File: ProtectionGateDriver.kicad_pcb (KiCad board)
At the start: 2 copper layers, 46.2 x 33.3 mm, 19 parts, among them J1 48V_INPUT_XT_MALE, J2 WHEEL_OUTPUT_XT_FEMALE, J3 12V_GATE_SUPPLY, J4 STM_CONTROL, Q1 MCTL1D0N08Y, U1 1EDN7550B

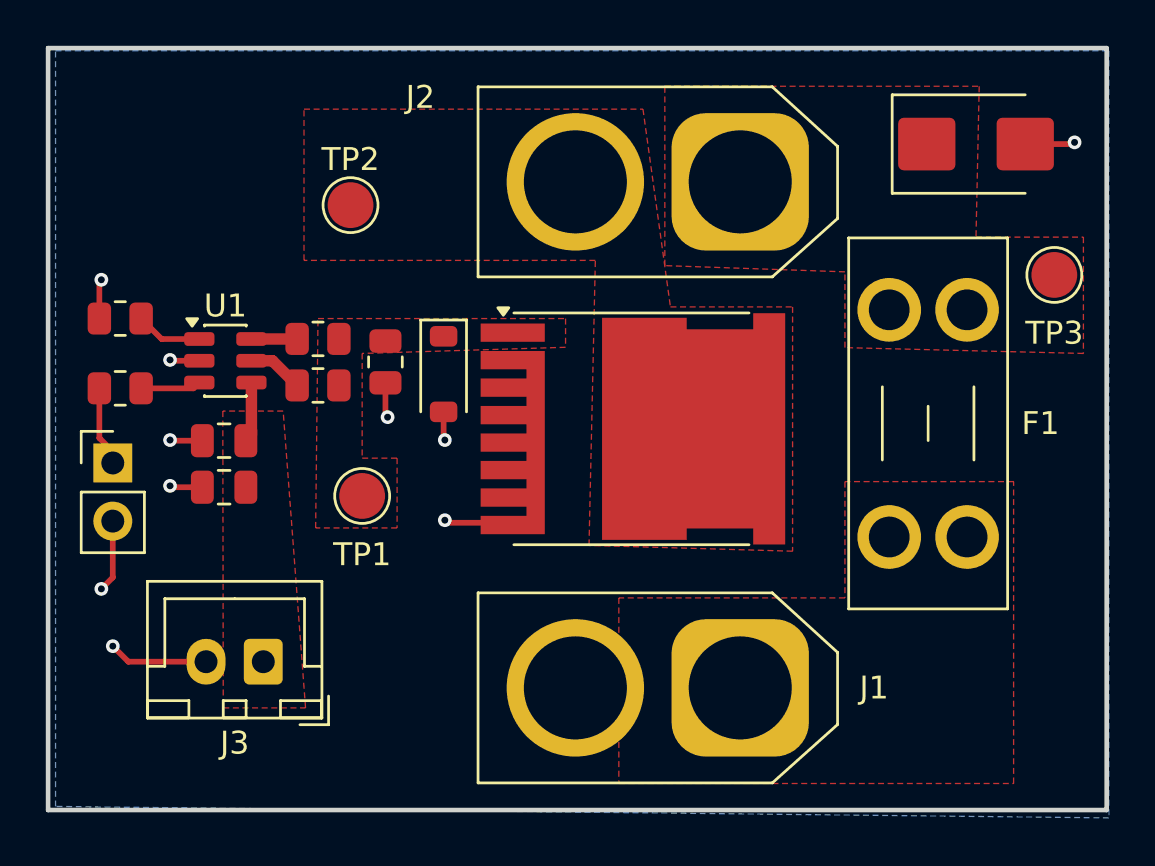
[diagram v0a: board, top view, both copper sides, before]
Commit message: Correct iteration 2 native KiCad files from uploaded project
Replace stale PCB, project and schematic with the supplied iteration 2 files. Four-layer layout is a review checkpoint, not for fabrication.
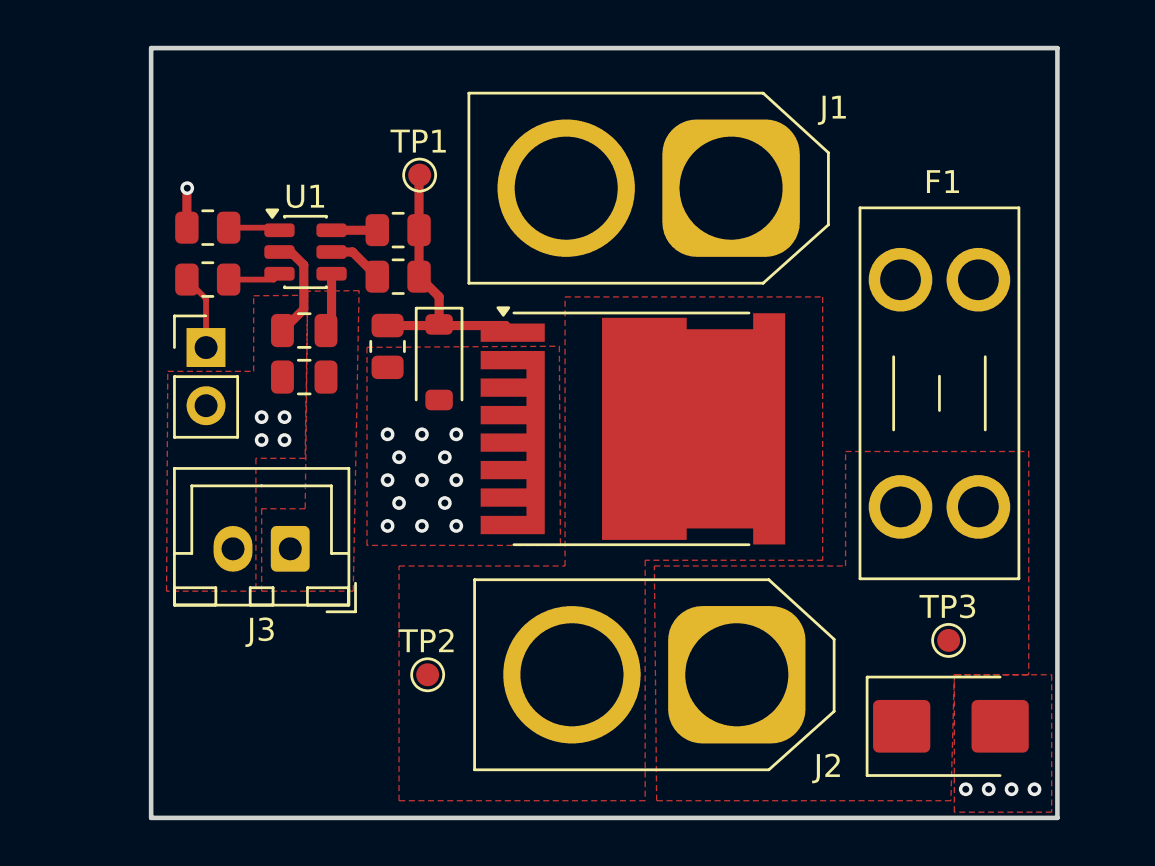
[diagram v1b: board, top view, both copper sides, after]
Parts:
- TP1, TP2, TP3: footprint TestPoint:TestPoint_Pad_D2.0mm -> TestPoint:TestPoint_Pad_D1.0mm
- moved D2 25.4 mm to (161.6, 109.5)
- moved J1 21.8 mm to (152.0, 86.0)
- moved J2 21.5 mm to (152.2, 107.2)
- moved TP2 20.8 mm to (138.8, 107.2)
- moved TP3 16.6 mm to (161.5, 105.8)
- moved TP1 14.2 mm to (138.4, 85.4)
- moved F1 11.9 mm to (162.8, 90.0), turned to -90 degrees
- moved J4 6.48 mm to (129.1, 93.0)
- moved R1 6.10 mm to (129.1, 90.0)
- moved C1 5.95 mm to (133.4, 92.2)
- moved C2 5.95 mm to (133.4, 94.2)
- moved R3 5.90 mm to (137.5, 89.9)
- moved R4 5.90 mm to (137.5, 87.8)
- moved U1 5.90 mm to (133.4, 88.8)
- moved R2 5.51 mm to (129.1, 87.7)
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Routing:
- net GND: track 22.4 -> 6.28 mm, vias 10 -> 22
- net /Q1_GATE: track 0.00 -> 12.5 mm
- net Net-(U1-IN-): track 2.91 -> 2.26 mm
- added copper zone on In2.Cu, net +48V
- added copper zone on F.Cu, net GND
- added copper zone on In1.Cu, net GND
- removed copper zone on F.Cu, net +48V
- removed copper zone on F.Cu, net /Q1_GATE
- removed copper zone on B.Cu, net GND
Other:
- board size 46.2 x 33.3 mm -> 39.6 x 33.6 mm
- copper layers 2 -> 4
